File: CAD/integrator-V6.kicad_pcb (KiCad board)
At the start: 2 copper layers, 80 x 47 mm, 37 parts, among them J1 Screw_Terminal_01x03, J2 Barrel_Jack_Switch, J3 AudioJack2_Ground_Switch, SW1 SW_SPDT_MSM, U1 TL084, U2 L78L06_SOT89

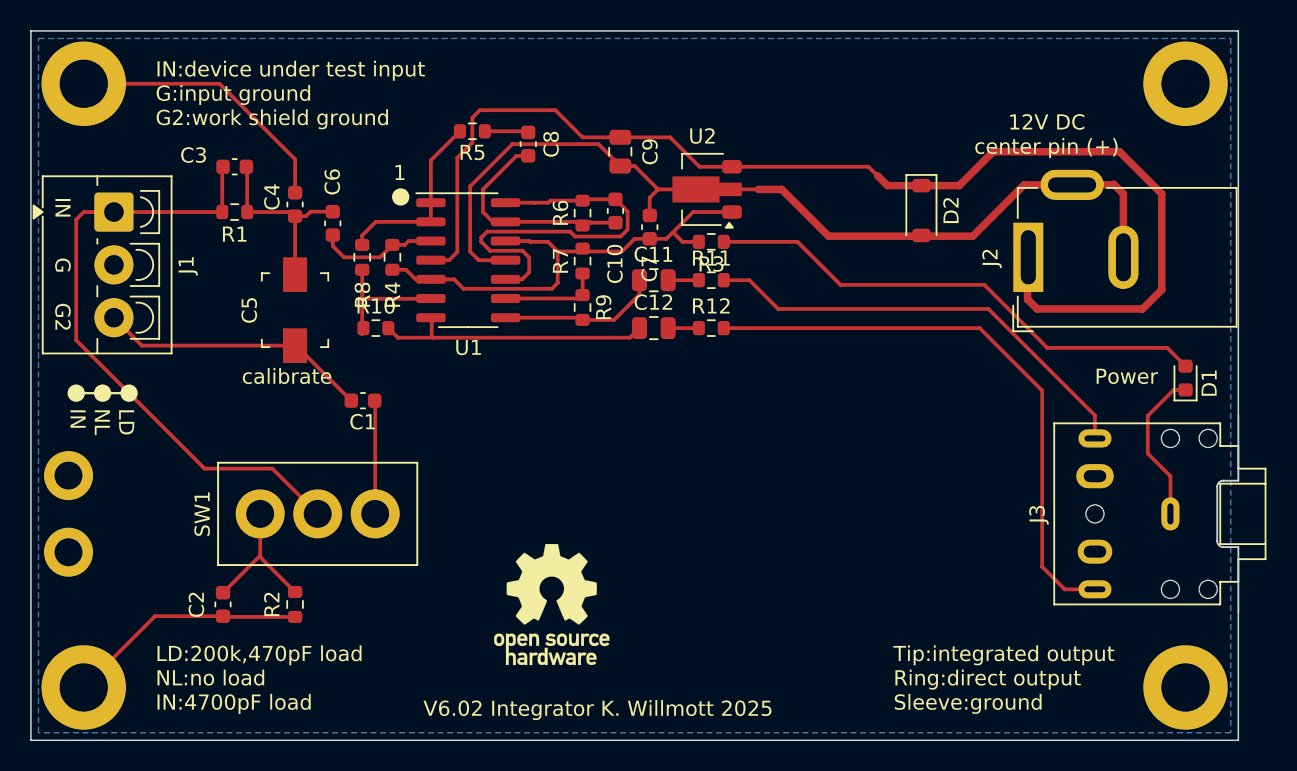
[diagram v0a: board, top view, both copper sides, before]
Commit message: Add files via upload
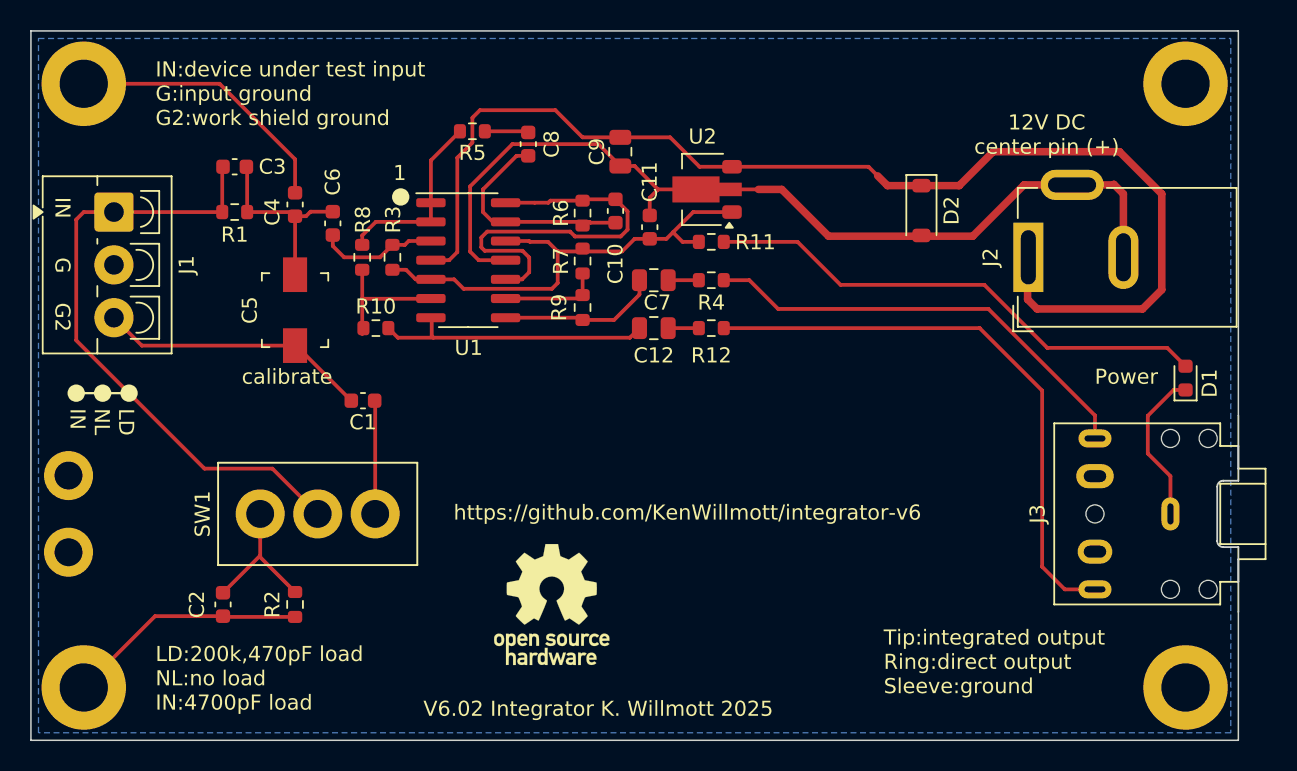
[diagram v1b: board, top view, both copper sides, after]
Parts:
- renumbered R4 to R3, R3 to R4
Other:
- board text added: "https://github.com/KenWillmott/integrator-v6"
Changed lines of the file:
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@@
 			(crossoutdnponfab yes)
 			(subtractmaskfromsilk no)
-			(outputformat 4)
+			(outputformat 1)
 			(mirror no)
 			(drillshape 0)
@@
 		(tags "resistor")
 		(property "Reference" "R9"
-			(at 0 -1.43 90)
+			(at 0 1.55 90)
 			(layer "F.SilkS")
 			(effects
@@
 		(tags "capacitor")
 		(property "Reference" "C9"
-			(at 0 -2 90)
+			(at 0 1.55 90)
 			(layer "F.SilkS")
 			(effects
@@
 		(tags "capacitor")
 		(property "Reference" "C12"
-			(at 0 -1.68 0)
+			(at 0 1.81 0)
 			(layer "F.SilkS")
 			(effects
@@
 		(tags "capacitor")
 		(property "Reference" "C11"
-			(at 0 -1.68 0)
+			(at -0.27 -6.515 90)
 			(layer "F.SilkS")
 			(effects
@@
 		(tags "resistor")
 		(property "Reference" "R11"
-			(at 0 -1.43 0)
+			(at 2.92 -2.515 0)
 			(layer "F.SilkS")
 			(effects
@@
 		(tags "capacitor")
 		(property "Reference" "C7"
-			(at -2.75 0 90)
+			(at -5 0.5 0)
 			(layer "F.SilkS")
 			(effects
@@
 		(descr "Resistor SMD 0603 (1608 Metric), square (rectangular) end terminal, IPC_7351 nominal, (Body size source: IPC-SM-782 page 72, https://www.pcb-3d.com/wordpress/wp-content/uploads/ipc-sm-782a_amendment_1_and_2.pdf), generated with kicad-footprint-generator")
 		(tags "resistor")
-		(property "Reference" "R3"
-			(at 0 1.5 0)
+		(property "Reference" "R4"
+			(at 0 4.025 0)
 			(layer "F.SilkS")
 			(effects
@@
 		(tags "capacitor")
 		(property "Reference" "C4"
-			(at -0.5 1.5 90)
+			(at 0.5 1.5 90)
 			(layer "F.SilkS")
 			(effects
@@
 		(tags "resistor")
 		(property "Reference" "R8"
-			(at 2.5 -0.05 90)
+			(at -2.5 -0.05 90)
 			(layer "F.SilkS")
 			(effects
@@
 		(descr "Resistor SMD 0603 (1608 Metric), square (rectangular) end terminal, IPC_7351 nominal, (Body size source: IPC-SM-782 page 72, https://www.pcb-3d.com/wordpress/wp-content/uploads/ipc-sm-782a_amendment_1_and_2.pdf), generated with kicad-footprint-generator")
 		(tags "resistor")
-		(property "Reference" "R4"
-			(at 2.5 -0.05 90)
+		(property "Reference" "R3"
+			(at -2.5 -0.05 90)
 			(layer "F.SilkS")
 			(effects
@@
 		(tags "capacitor")
 		(property "Reference" "C3"
-			(at -2.71 -0.74 0)
+			(at 2.5 0 0)
 			(layer "F.SilkS")
 			(effects
@@
 		(tags "resistor")
 		(property "Reference" "R12"
-			(at 0 -1.43 0)
+			(at 0 1.81 0)
 			(layer "F.SilkS")
 			(effects
@@
 	)
 	(gr_text "Tip:integrated output\nRing:direct output\nSleeve:ground"
-		(at 157.145 121.59 0)
+		(at 156.5 120.5 0)
 		(layer "F.SilkS")
 		(effects
@@
 		)
 	)
+	(gr_text "https://github.com/KenWillmott/integrator-v6"
+		(at 128 109 0)
+		(layer "F.SilkS")
+		(effects
+			(font
+				(size 1 1)
+				(thickness 0.15)
+			)
+			(justify left bottom)
+		)
+	)
 	(gr_text "Power"
 		(at 170.48 100 0)
@@
 	)
 	(segment
-		(start 130.232 89.794)
-		(end 129.84 90.186)
-		(width 0.25)
-		(layer "F.Cu")
-		(net 2)
-	)
-	(segment
-		(start 130.429 91.064)
-		(end 132.564 91.064)
+		(start 132.54 92.96)
+		(end 131.45 92.96)
 		(width 0.25)
 		(layer "F.Cu")
@@
 	)
 	(segment
-		(start 132.564 91.064)
-		(end 133.015 91.515)
+		(start 133.015 91.515)
+		(end 133.015 92.485)
 		(width 0.25)
 		(layer "F.Cu")
@@
 	)
 	(segment
-		(start 135.724582 89.794)
-		(end 130.232 89.794)
+		(start 134.285 87.88)
+		(end 134.42 87.745)
 		(width 0.25)
 		(layer "F.Cu")
@@
 	)
 	(segment
-		(start 134.285 87.88)
-		(end 134.42 87.745)
+		(start 139.531 88.456)
+		(end 139.531 89.664466)
 		(width 0.25)
 		(layer "F.Cu")
@@
 	)
 	(segment
-		(start 139.531 89.664466)
-		(end 139.074466 90.121)
+		(start 134.42 87.745)
+		(end 136.55 87.745)
 		(width 0.25)
 		(layer "F.Cu")
@@
 	)
 	(segment
-		(start 133.015 91.515)
-		(end 133.015 92.485)
+		(start 136.64 87.655)
+		(end 138.73 87.655)
 		(width 0.25)
 		(layer "F.Cu")
@@
 	)
 	(segment
-		(start 138.73 87.655)
-		(end 139.531 88.456)
+		(start 136.051582 90.121)
+		(end 135.724582 89.794)
 		(width 0.25)
 		(layer "F.Cu")
@@
 	)
 	(segment
-		(start 134.42 87.745)
-		(end 136.55 87.745)
+		(start 133.38 87.88)
+		(end 134.285 87.88)
 		(width 0.25)
 		(layer "F.Cu")
@@
 	)
 	(segment
-		(start 132.54 92.96)
-		(end 131.45 92.96)
+		(start 135.724582 89.794)
+		(end 130.232 89.794)
 		(width 0.25)
 		(layer "F.Cu")
@@
 	)
 	(segment
-		(start 129.84 90.475)
-		(end 130.429 91.064)
+		(start 136.55 87.745)
+		(end 136.64 87.655)
 		(width 0.25)
 		(layer "F.Cu")
@@
 	)
 	(segment
-		(start 136.051582 90.121)
-		(end 135.724582 89.794)
+		(start 139.074466 90.121)
+		(end 136.051582 90.121)
 		(width 0.25)
 		(layer "F.Cu")
@@
 	(segment
 		(start 129.84 90.186)
-		(end 129.84 90.475)
+		(end 129.84 90.84)
 		(width 0.25)
 		(layer "F.Cu")
@@
 	)
 	(segment
-		(start 136.64 87.655)
-		(end 138.73 87.655)
+		(start 129.84 90.84)
+		(end 130.064 91.064)
 		(width 0.25)
 		(layer "F.Cu")
@@
 	)
 	(segment
-		(start 133.38 87.88)
-		(end 134.285 87.88)
+		(start 132.564 91.064)
+		(end 133.015 91.515)
 		(width 0.25)
 		(layer "F.Cu")
@@
 	)
 	(segment
-		(start 136.55 87.745)
-		(end 136.64 87.655)
+		(start 139.531 89.664466)
+		(end 139.074466 90.121)
 		(width 0.25)
 		(layer "F.Cu")
@@
 	)
 	(segment
-		(start 139.531 88.456)
-		(end 139.531 89.664466)
+		(start 130.064 91.064)
+		(end 132.564 91.064)
 		(width 0.25)
 		(layer "F.Cu")
@@
 	)
 	(segment
-		(start 139.074466 90.121)
-		(end 136.051582 90.121)
+		(start 138.73 87.655)
+		(end 139.531 88.456)
 		(width 0.25)
 		(layer "F.Cu")
@@
 		(width 0.25)
 		(layer "F.Cu")
+		(net 2)
+	)
+	(segment
+		(start 130.232 89.794)
+		(end 129.84 90.186)
+		(width 0.25)
+		(layer "F.Cu")
